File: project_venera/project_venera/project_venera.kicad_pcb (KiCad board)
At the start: 2 copper layers, 2 parts, among them IC1 ATSAMD11D14A-SSUT, IC2 TC1262-3.3VDBTR

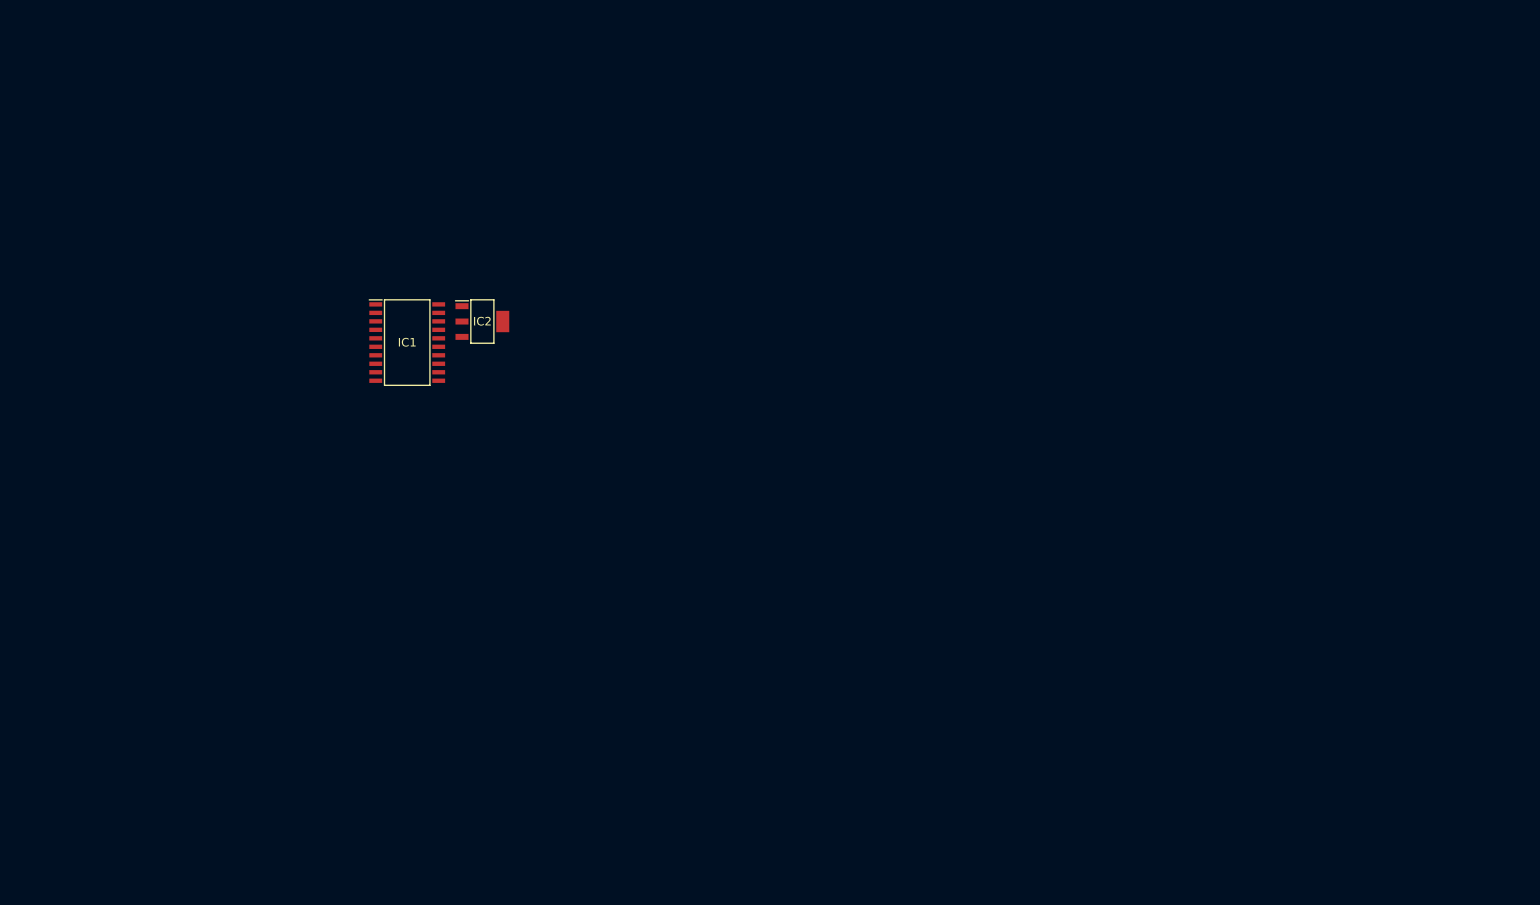
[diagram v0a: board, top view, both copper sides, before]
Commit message: progress on board
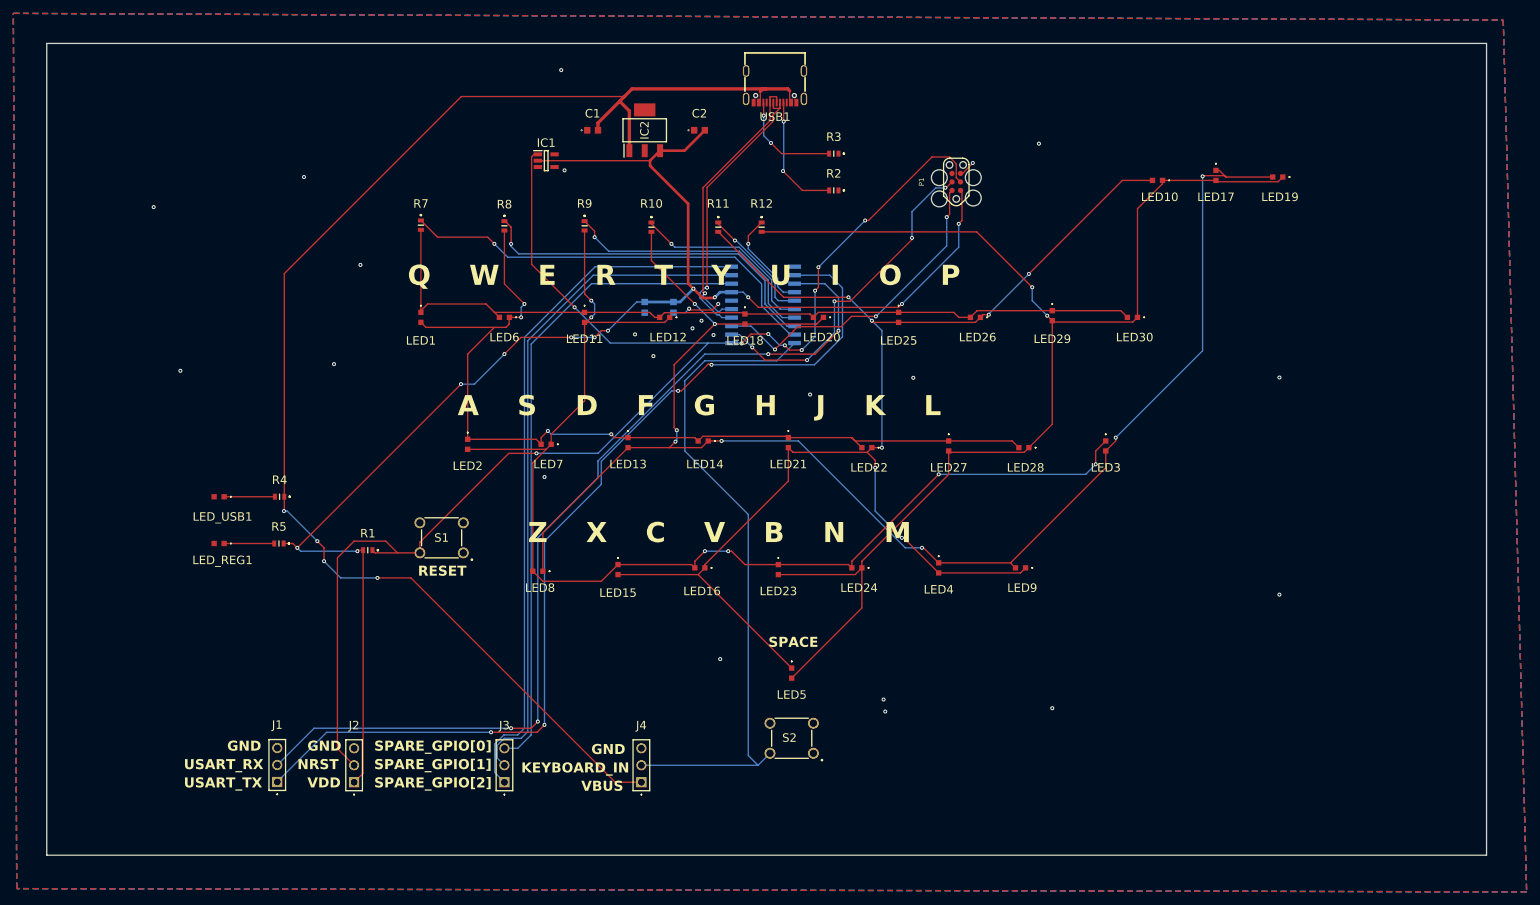
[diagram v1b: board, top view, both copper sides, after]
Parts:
- added C1: 1uF, LibraryLoader:C0603, F.Cu at (120.7, 43.5)
- added C2: 1uF, LibraryLoader:C0603, F.Cu at (136.7, 43.5)
- added C3: 100nF, LibraryLoader:C0603, B.Cu at (132.8, 70.0)
- added C4: 4.7uF, LibraryLoader:C0603, B.Cu at (128.5, 70.0)
- added IC1: NCV303LSN11T1G, LibraryLoader:SOT95P275X110-5N, F.Cu at (113.8, 48.0)
- added J1: 0022285034, LibraryLoader:0022285034, F.Cu at (73.5, 141.0)
- added J2: 0022285034, LibraryLoader:0022285034, F.Cu at (85.0, 141.1)
- added J3: 0022285034, LibraryLoader:0022285034, F.Cu at (107.5, 141.1)
- added J4: 0022285034, LibraryLoader:0022285034, F.Cu at (128.0, 141.1)
- added LED1: SM0603SRC, LibraryLoader:SM0603SRC, F.Cu at (95.0, 71.5)
- added LED10: SM0603SRC, LibraryLoader:SM0603SRC, F.Cu at (205.2, 51.0)
- added LED11: SM0603SRC, LibraryLoader:SM0603SRC, F.Cu at (119.5, 71.5)
- added LED12: SM0603SRC, LibraryLoader:SM0603SRC, F.Cu at (131.5, 71.5)
- added LED13: SM0603SRC, LibraryLoader:SM0603SRC, F.Cu at (126.0, 90.2)
- added LED14: SM0603SRC, LibraryLoader:SM0603SRC, F.Cu at (137.2, 90.0)
- added LED15: SM0603SRC, LibraryLoader:SM0603SRC, F.Cu at (124.5, 109.2)
- added LED16: SM0603SRC, LibraryLoader:SM0603SRC, F.Cu at (136.8, 109.0)
- added LED17: SM0603SRC, LibraryLoader:SM0603SRC, F.Cu at (214.0, 50.2)
- added LED18: SM0603SRC, LibraryLoader:SM0603SRC, F.Cu at (143.5, 71.8)
- added LED19: SM0603SRC, LibraryLoader:SM0603SRC, F.Cu at (223.2, 50.5)
- added LED2: SM0603SRC, LibraryLoader:SM0603SRC, F.Cu at (102.0, 90.5)
- added LED20: SM0603SRC, LibraryLoader:SM0603SRC, F.Cu at (154.5, 71.5)
- added LED21: SM0603SRC, LibraryLoader:SM0603SRC, F.Cu at (150.0, 90.2)
- added LED22: SM0603SRC, LibraryLoader:SM0603SRC, F.Cu at (161.8, 91.0)
- added LED23: SM0603SRC, LibraryLoader:SM0603SRC, F.Cu at (148.5, 109.2)
- added LED24: SM0603SRC, LibraryLoader:SM0603SRC, F.Cu at (160.2, 109.0)
- added LED25: SM0603SRC, LibraryLoader:SM0603SRC, F.Cu at (166.5, 71.5)
- added LED26: SM0603SRC, LibraryLoader:SM0603SRC, F.Cu at (178.0, 71.5)
- added LED27: SM0603SRC, LibraryLoader:SM0603SRC, F.Cu at (174.0, 90.8)
- added LED28: SM0603SRC, LibraryLoader:SM0603SRC, F.Cu at (185.2, 91.0)
- added LED29: SM0603SRC, LibraryLoader:SM0603SRC, F.Cu at (189.5, 71.2)
- added LED3: SM0603SRC, LibraryLoader:SM0603SRC, F.Cu at (197.5, 90.8)
- added LED30: SM0603SRC, LibraryLoader:SM0603SRC, F.Cu at (201.5, 71.5)
- added LED4: SM0603SRC, LibraryLoader:SM0603SRC, F.Cu at (172.5, 109.0)
- added LED5: SM0603SRC, LibraryLoader:SM0603SRC, F.Cu at (150.5, 124.8)
- added LED6: SM0603SRC, LibraryLoader:SM0603SRC, F.Cu at (107.5, 71.5)
- added LED7: SM0603SRC, LibraryLoader:SM0603SRC, F.Cu at (113.8, 90.5)
- added LED8: SM0603SRC, LibraryLoader:SM0603SRC, F.Cu at (112.5, 109.5)
- added LED9: SM0603SRC, LibraryLoader:SM0603SRC, F.Cu at (184.8, 109.0)
- added LED_REG1: SM0603SRC, LibraryLoader:SM0603SRC, F.Cu at (64.8, 105.3)
- added LED_USB1: SM0603SRC, LibraryLoader:SM0603SRC, F.Cu at (64.8, 98.3)
- added P1: TC2030-CTX, TagConnect:TC2030_SMALL, F.Cu at (175.1, 51.2)
- added R1: 10K, LibraryLoader:ERJPC3D9763V, F.Cu at (87.0, 106.3)
- added R10: TBD, LibraryLoader:ERJPC3D9763V, F.Cu at (129.5, 58.0)
- added R11: TBD, LibraryLoader:ERJPC3D9763V, F.Cu at (139.5, 58.0)
- added R12: TBD, LibraryLoader:ERJPC3D9763V, F.Cu at (146.0, 58.0)
- added R2: 5.1K, LibraryLoader:ERJPC3D9763V, F.Cu at (156.8, 52.5)
- added R3: 5.1K, LibraryLoader:ERJPC3D9763V, F.Cu at (156.8, 47.0)
- added R4: TBD, LibraryLoader:ERJPC3D9763V, F.Cu at (73.8, 98.3)
- added R5: TBD, LibraryLoader:ERJPC3D9763V, F.Cu at (73.8, 105.3)
- added R7: TBD, LibraryLoader:ERJPC3D9763V, F.Cu at (95.0, 57.7)
- added R8: TBD, LibraryLoader:ERJPC3D9763V, F.Cu at (107.5, 57.8)
- added R9: TBD, LibraryLoader:ERJPC3D9763V, F.Cu at (119.5, 57.8)
- added S1: B3F-1020, LibraryLoader:B3F1000, F.Cu at (98.1, 104.5)
- added S2: B3F-1020, LibraryLoader:B3F1000, F.Cu at (150.5, 134.5)
- added USB1: USB4105-GF-A-060, CustomLib:USB-C-SMD_GT-USB-7010E-1, F.Cu at (148.0, 37.0)
- IC3: renamed from IC1; moved to B.Cu
- moved IC3 53.6 mm to (146.2, 69.6), turned to 180 degrees
- moved IC2 37.5 mm to (128.5, 43.5), turned to 90 degrees
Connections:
- IC2 pad 1: unconnected-(IC2-VIN-Pad1) -> /VBUS
- IC2 pad 2: unconnected-(IC2-GND_1-Pad2) -> GND
- IC2 pad 3: unconnected-(IC2-VOUT-Pad3) -> VDD
- IC2 pad 4: unconnected-(IC2-GND_2-Pad4) -> GND
- IC3 pad 10: unconnected-(IC1-PA23-Pad10) -> /KEYBOARD_IN
- IC3 pad 11: unconnected-(IC1-PA28/~{RST}-Pad11) -> /NRST
- IC3 pad 12: unconnected-(IC1-PA30-Pad12) -> /SWCLK
- IC3 pad 13: unconnected-(IC1-PA31-Pad13) -> /SWDIO
- IC3 pad 14: unconnected-(IC1-PA24-Pad14) -> /DP-
- IC3 pad 15: unconnected-(IC1-PA25-Pad15) -> /DP+
- IC3 pad 17: unconnected-(IC1-VDDIO/IN/ANA-Pad17) -> VDD
- IC3 pad 18: unconnected-(IC1-PA02-Pad18) -> /SPARE_GPIO[0]
- IC3 pad 19: unconnected-(IC1-PA03-Pad19) -> /SPARE_GPIO[1]
- IC3 pad 2: unconnected-(IC1-PA06-Pad2) -> /USART_TX
- IC3 pad 20: unconnected-(IC1-PA04-Pad20) -> /SPARE_GPIO[2]
- IC3 pad 3: unconnected-(IC1-PA07-Pad3) -> /USART_RX
- IC3 pad 4: unconnected-(IC1-PA08-Pad4) -> /LED Array/CHARLIEPLEXING_5
- IC3 pad 5: unconnected-(IC1-PA09-Pad5) -> /LED Array/CHARLIEPLEXING_4
- IC3 pad 6: unconnected-(IC1-PA14-Pad6) -> /LED Array/CHARLIEPLEXING_3
- IC3 pad 7: unconnected-(IC1-PA15-Pad7) -> /LED Array/CHARLIEPLEXING_2
- IC3 pad 8: unconnected-(IC1-PA16-Pad8) -> /LED Array/CHARLIEPLEXING_1
- IC3 pad 9: unconnected-(IC1-PA22-Pad9) -> /LED Array/CHARLIEPLEXING_0
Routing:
- net Net-(LED13-K): track 0.00 -> 228.4 mm, vias 0 -> 8
- net VDD: track 0.00 -> 225.9 mm, vias 0 -> 12
- net /NRST: track 0.00 -> 215.6 mm, vias 0 -> 9
- net /VBUS: track 0.00 -> 213.5 mm, vias 0 -> 4
- net Net-(LED10-K): track 0.00 -> 206.0 mm, vias 0 -> 7
- net Net-(LED10-A): track 0.00 -> 193.2 mm, vias 0 -> 2
- net Net-(LED11-K): track 0.00 -> 180.3 mm, vias 0 -> 6
- net /USART_TX: track 0.00 -> 145.7 mm, vias 0 -> 4
- net /USART_RX: track 0.00 -> 140.9 mm, vias 0 -> 4
- net Net-(LED1-K): track 0.00 -> 137.3 mm, vias 0 -> 4
- net Net-(LED1-A): track 0.00 -> 122.7 mm
- net /SPARE_GPIO[2]: track 0.00 -> 105.6 mm
- net /SPARE_GPIO[1]: track 0.00 -> 101.9 mm
- net /KEYBOARD_IN: track 0.00 -> 100.8 mm
- net /SPARE_GPIO[0]: track 0.00 -> 97.1 mm
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- added copper zone on B.Cu, net GND
- added copper zone on F.Cu, net GND
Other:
- board outline added: 215.5 x 121.5 mm
- board text added: "A S D F G H J K L"
- board text added: "GND"
- board text added: "KEYBOARD_IN"
- board text added: "NRST"
- board text added: "Q W E R T Y U I O P"
- board text added: "RESET"
- board text added: "SPACE"
- board text added: "SPARE_GPIO[0]"
- board text added: "SPARE_GPIO[1]"
- board text added: "SPARE_GPIO[2]"
- board text added: "USART_RX"
- board text added: "USART_TX"
- board text added: "VBUS"
- board text added: "VDD"
- board text added: "Z X C V B N M"
